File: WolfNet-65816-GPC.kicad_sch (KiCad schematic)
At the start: 4 parts, among them U1 WD65C816S, U2 AS6C8008, U3 28C040, U4 28C040

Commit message: Update WolfNet-65816-GPC.kicad_sch
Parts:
- removed U2: AS6C8008, symbol Memory:AS6C8008
- added SW1: SW_Push, symbol Switch:SW_Push
- added U5: 74HCT573, symbol 74xx:74LS573
- added U6: 74HCT245, symbol 74xx:74HC245
- added U7: 22V10, symbol GALs:22V10
- added U8: XCR3064XL-VQ100, Package_QFP:LQFP-100_14x14mm_P0.5mm, symbol CPLD_Xilinx:XCR3064XL-VQ100
- added U9: DS1813, symbol Supervisory Circuit:DS1813
- added U?: AS6C1608, symbol Memory:AS6C1608
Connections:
- net A0: now also U8.85 (A0), U?.5 (A0)
- net A1: now also U8.84 (A1), U?.4 (A1)
- net A10: now also U8.69 (A10), U?.27 (A10)
- net A11: now also U8.68 (A11), U?.26 (A11)
- net A12: now also U8.67 (A12), U?.25 (A12)
- net A13: now also U8.65 (A13), U?.24 (A13)
- net A14: now also U8.64 (A14), U?.23 (A14)
- net A15: now also U8.63 (A15), U?.22 (A15)
- net A16: now also U5.19 (Q0), U8.92 (B0), U?.21 (A16)
- net A17: now also U5.18 (Q1), U8.93 (B1), U?.20 (A17)
- net A18: now also U5.17 (Q2), U8.94 (B2), U?.19 (A18)
- net A19: now also U5.16 (Q3), U8.96 (B3), U?.18 (A19)
- net A2: now also U8.83 (A2), U?.3 (A2)
- net A3: now also U8.81 (A3), U?.2 (A3)
- net A4: now also U8.80 (A4), U?.1 (A4)
- net A5: now also U8.79 (A5), U?.44 (A5)
- net A6: now also U8.76 (A6), U?.43 (A6)
- net A7: now also U8.75 (A7), U?.42 (A7)
- net A8: now also U8.73 (A8/TDO), U?.39 (A8)
- net A9: now also U8.71 (A9), U?.28 (A9)
- net D0: now also U6.2 (A0), U?.9 (DQ0)
- net D1: now also U6.3 (A1), U?.10 (DQ1)
- net D2: now also U6.4 (A2), U?.13 (DQ2)
- net D3: now also U6.5 (A3), U?.14 (DQ3)
- net D4: now also U6.6 (A4), U?.31 (DQ4)
- net D5: now also U6.7 (A5), U?.32 (DQ5)
- net D6: now also U6.8 (A6), U?.35 (DQ6)
- net D7: now also U?.36 (DQ7)
- net DA0: now also U5.2 (D0), U6.18 (B0)
- net DA1: now also U5.3 (D1), U6.17 (B1)
- net DA2: now also U5.4 (D2), U6.16 (B2)
- net DA3: now also U5.5 (D3), U6.15 (B3)
- net DA4: now also U5.6 (D4), U6.14 (B4)
- net DA5: now also U5.7 (D5), U6.13 (B5)
- net DA6: now also U5.8 (D6), U6.12 (B6)
- net DA7: now also U5.9 (D7), U6.11 (B7)
- net GND: now also SW1.2, U5.1 (OE), U5.10 (GND), U6.10 (GND), U7.12 (GND), U8.26 (GND), U8.38 (GND), U8.43 (GND), U8.59 (GND), U8.74 (GND), U8.86 (GND), U8.95 (GND), U9.3 (GND), U?.12 (GND), U?.34 (GND)
- net RAM_CE2: now also U?.40 (CE2)
- net R/~{W}: now also U6.1 (A->B), U7.2 (IN)
- net ~{RAM_EN}: now also U?.6 (~{CE})
- net ~{RAM_OE}: now also U?.41 (~{OE})
- net ~{RAM_WE}: now also U?.17 (~{WE})
- net ~{RESET}: now also SW1.1, U9.1 (~{RST})
- net VCC renamed +5V
- net +5V: now also U5.20 (VCC), U6.20 (VCC), U7.24 (VCC), U8.18 (VCC), U8.3 (VCC), U8.34 (VCC), U8.39 (VCC), U8.51 (VCC), U8.66 (VCC), U8.82 (VCC), U8.91 (VCC), U9.2 (VCC), U?.11 (VCC), U?.33 (VCC)
- new net A20: U5.15 (Q4), U8.97 (B4), U?.16 (A20)
- new net A21: U5.14 (Q5), U8.98 (B5)
- new net A22: U5.13 (Q6), U8.99 (B6)
- new net A23: U5.12 (Q7), U8.100 (B7)
- new net D8: U6.9 (A7)
- new net DecoderJTAG: U8.11 (PORT_EN)
- new net NOT_PHI2: U5.11 (Load), U6.19 (CE), U7.23 (I/O)
- new net PHI2: U7.1 (CLK/IN), U8.90 (CLK0/IN0)
- new net READ: U7.22 (I/O)
- new net WRITE: U7.21 (I/O)
- no-connect marks 8 -> 7
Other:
- note added: "Address Decoding"
- note added: "Bank Address Latch"
- note added: "Direct Memory Access Circuit"
- note added: "Memory Management"
- note added: "Supervisory Circuit"

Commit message: Almost there...
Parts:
- added D?: PWR_OK1, symbol Device:LED
- added J1: ATX-24, symbol Connector:ATX-24
- added R?: 220 Ω, symbol Device:R
- added R?: PWR220T-20-5R00J, symbol Device:R
- added SW1: SW_SPST, symbol Switch:SW_SPST
- added U5: XCR3064XL-VQ100, Package_QFP:LQFP-100_14x14mm_P0.5mm, symbol CPLD_Xilinx:XCR3064XL-VQ100
- added U?: SC28L91, symbol UART:SC28L91
- added U?: MCP2200-I-SO, Package_SO:SOIC-20W_7.5x12.8mm_P1.27mm, symbol Interface_USB:MCP2200-I-SO
- gave numbers to parts that had none: 1
- renumbered SW1 to SW2, U9 to U10, U5 to U2, U6 to U3, U3 to U6, U4 to U7, U7 to U8, U8 to U9
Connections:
- net +5V: now also J1.21 (+5V), J1.22 (+5V), J1.23 (+5V), J1.4 (+5V), J1.6 (+5V), R?.1, U5.18 (VCC), U5.3 (VCC), U5.34 (VCC), U5.39 (VCC), U5.51 (VCC), U5.66 (VCC), U5.82 (VCC), U5.91 (VCC), U?.11 (VCC), U?.12 (MODE_SELECT), U?.44 (VCC)
- net A0: now also U?.2 (A0)
- net A1: now also U?.4 (A1)
- net A2: now also U?.6 (A2)
- net A3: now also U?.7 (A3)
- net GND: now also D?.1 (K), J1.15 (GND), J1.17 (GND), J1.18 (GND), J1.19 (GND), J1.24 (GND), J1.3 (GND), J1.5 (GND), J1.7 (GND), R?.2, SW1.1 (A), U5.26 (GND), U5.38 (GND), U5.43 (GND), U5.59 (GND), U5.74 (GND), U5.86 (GND), U5.95 (GND), U?.22 (GND)
- net PHI2: now also U5.90 (CLK0/IN0)
- net ~{RESET}: now also U?.4 (RST)
- net READ renamed ~{READ}
- net ~{READ}: now also U?.10 (~{RD})
- net WRITE renamed ~{WRITE}
- net ~{WRITE}: now also U?.9 (~{WR})
- new net: J1.8 (PWR_OK), R?.1
- new net: D?.2 (A), R?.2
- new net: J1.1 (+3.3V), J1.12 (+3.3V), J1.13 (+3.3V), J1.2 (+3.3V)
- new net: J1.16 (PS_ON#), SW1.2 (B)
- new net +12V: J1.10 (+12V), J1.11 (+12V)
- new net -12V: J1.14 (-12V)
- new net DMA_JTAG: U5.11 (PORT_EN)
- no-connect marks 7 -> 9
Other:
- note added: "ATX power connector"
- note added: "UART"
- note added: "USB Connection"

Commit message: Update WolfNet-65816-GPC.kicad_sch
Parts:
- removed U8: 22V10, symbol GALs:22V10
- added C?: 10 µF, symbol Device:C
- added D? (x2): GREEN, symbol Device:LED
- added J? (x4): Conn_01x01, symbol Connector_Generic:Conn_01x01
- added R? (x2): R, symbol Device:R
- added X?: ACO-12MHz, Oscillator:Oscillator_DIP-14, symbol Oscillator:ACO-xxxMHz
- added X?: ACO-xxxMHz, Oscillator:Oscillator_DIP-14, symbol Oscillator:ACO-xxxMHz
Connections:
- net +5V: now also X?.14 (Vcc), X?.14 (Vcc)
- net A8: now also J?.1 (Pin_1)
- net D0: now also U?.28 (D0)
- net D1: now also U?.18 (D1)
- net D2: now also U?.27 (D2)
- net D3: now also U?.19 (D3)
- net D4: now also U?.26 (D4)
- net D5: now also U?.20 (D5)
- net D6: now also U?.25 (D6)
- net D7: now also U?.21 (D7)
- net GND: now also U?.20 (VSS), C?.1, D?.1 (K), D?.1 (K), X?.7 (GND), X?.7 (GND)
- net NOT_PHI2: now also U9.4 (B8/TDI), J?.1 (Pin_1)
- net R/~{W}: now also U9.9 (B11); no longer U3.1 (A->B)
- net ~{IRQ}: now also U?.24 (~{IRQ})
- net ~{RAM_EN}: now also U9.37 (D15)
- net ~{READ}: now also U9.10 (B12)
- net ~{RESET}: now also U?.38 (RESET)
- net ~{WRITE}: now also U3.1 (A->B), U9.12 (B13)
- net at U9.15 (D0/TMS): now also J?.1 (Pin_1)
- net ~{UART_EN}: now reaches U9.29 (D8)
- net ~{UART_EN}: now also U?.39 (~{CE})
- net ~{ROM2_EN}: now reaches U9.31 (D10)
- net ~{ROM2_EN}: now also U7.22 (~{CE})
- net ~{ROM1_EN}: now reaches U9.33 (D12)
- net ~{ROM1_EN}: now also U6.22 (~{CE})
- net at U9.62 (C0/TCK): now also J?.1 (Pin_1)
- net TxD: now reaches U?.33 (TxD)
- net TxD: now also U?.12 (RX)
- net RxD: now reaches U?.35 (RxD)
- net RxD: now also U?.10 (TX)
- net at U?.36 (X1/CLK): now also X?.8 (OUT)
- net VBUS: now reaches U?.1 (VDD)
- net at U?.17 (V_USB): now also C?.2
- net USB_D-: now reaches U?.18 (D-)
- net USB_D+: now reaches U?.19 (D+)
- net at U?.2 (OSC1): now also X?.8 (OUT)
- net at U?.5 (GP7/TxLED): now also R?.1
- net at U?.6 (GP6/RxLED): now also R?.1
- net RAM_CE2 renamed RAM_EN2
- removed net ~{ROM_CE}: U6.22 (~{CE}), U7.22 (~{CE})
- net ~{ROM_OE} renamed ~{ROM1_OE}
- net ~{ROM1_OE}: no longer U7.24 (~{OE})
- new net: D?.2 (A), R?.2 (x2)
- new net ~{ROM2_OE}: U7.24 (~{OE})
- no-connect marks 9 -> 38
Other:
- note removed: "Memory Management"

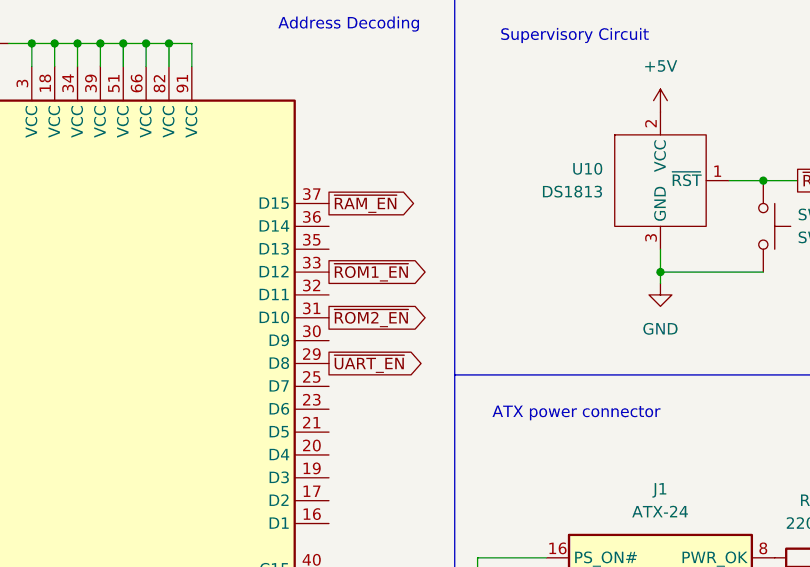
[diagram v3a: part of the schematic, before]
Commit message: Update WolfNet-65816-GPC.kicad_sch
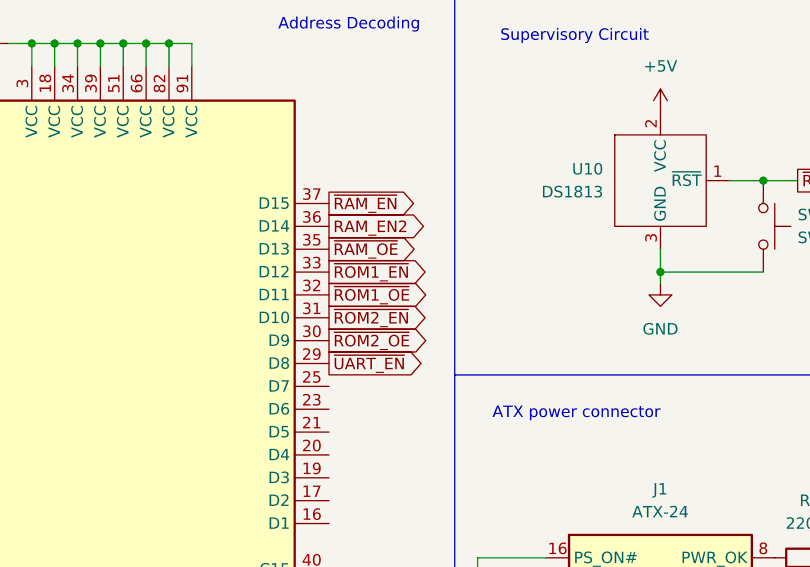
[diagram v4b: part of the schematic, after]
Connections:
- net RAM_EN2: now also U9.36 (D14)
- net ~{RAM_OE}: now also U9.35 (D13)
- net ~{ROM1_OE}: now also U9.32 (D11)
- net ~{ROM2_OE}: now also U9.30 (D9)
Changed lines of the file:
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@@
+    )
+  )
+  (global_label "RAM_EN2" (shape output) (at 336.55 109.22 0) (fields_autoplaced)
+    (effects (font (size 1.27 1.27)) (justify left))
+    (property "Intersheet References" "${INTERSHEET_REFS}" (id 0) (at 347.4298 109.1406 0)
+      (effects (font (size 1.27 1.27)) (justify left) hide)
     )
   )
@@
     )
   )
+  (global_label "~{ROM2_OE}" (shape output) (at 336.55 121.92 0) (fields_autoplaced)
+    (effects (font (size 1.27 1.27)) (justify left))
+    (property "Intersheet References" "${INTERSHEET_REFS}" (id 0) (at 347.6717 121.8406 0)
+      (effects (font (size 1.27 1.27)) (justify left) hide)
+    )
+  )
   (global_label "RxD" (shape output) (at 34.29 232.41 180) (fields_autoplaced)
     (effects (font (size 1.27 1.27)) (justify right))
@@
     )
   )
+  (global_label "~{RAM_OE}" (shape output) (at 336.55 111.76 0) (fields_autoplaced)
+    (effects (font (size 1.27 1.27)) (justify left))
+    (property "Intersheet References" "${INTERSHEET_REFS}" (id 0) (at 346.2202 111.6806 0)
+      (effects (font (size 1.27 1.27)) (justify left) hide)
+    )
+  )
   (global_label "A5" (shape input) (at 143.51 25.4 0) (fields_autoplaced)
     (effects (font (size 1.27 1.27)) (justify left))
@@
       (effects (font (size 1.27 1.27)) (justify left) hide)
     )
+  )
+  (global_label "~{ROM1_OE}" (shape output) (at 336.55 116.84 0) (fields_autoplaced)
+    (effects (font (size 1.27 1.27)) (justify left))
+    (property "Intersheet References" "${INTERSHEET_REFS}" (id 0) (at 347.6717 116.7606 0)
+      (effects (font (size 1.27 1.27)) (justify left) hide)
+    )
